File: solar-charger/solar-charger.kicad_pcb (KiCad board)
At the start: 2 copper layers, 20.8 x 10 mm, 11 parts, among them IC1 TLV809, IC2 TLV803, J1 solar, J2 battery, J3 out, Q1 AO3415, Q2 AO3416

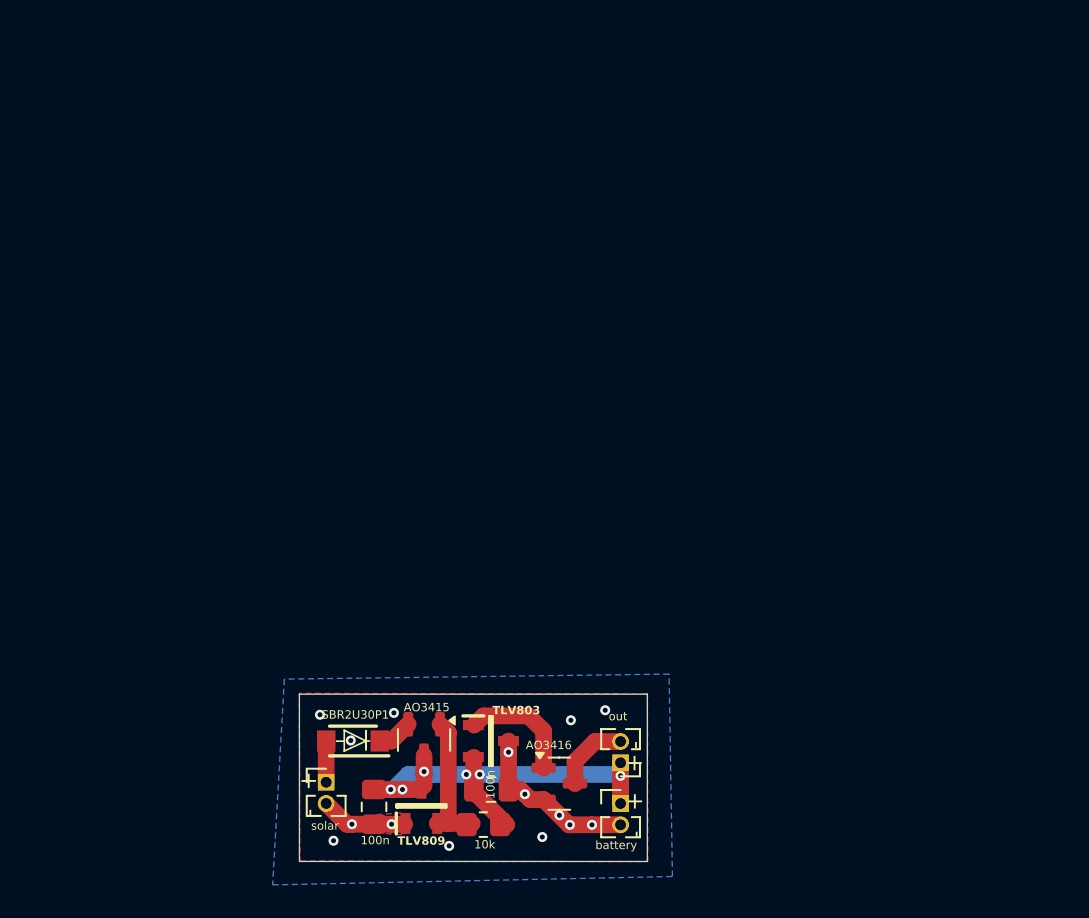
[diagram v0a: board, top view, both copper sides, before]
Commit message: finish 1. working PCB
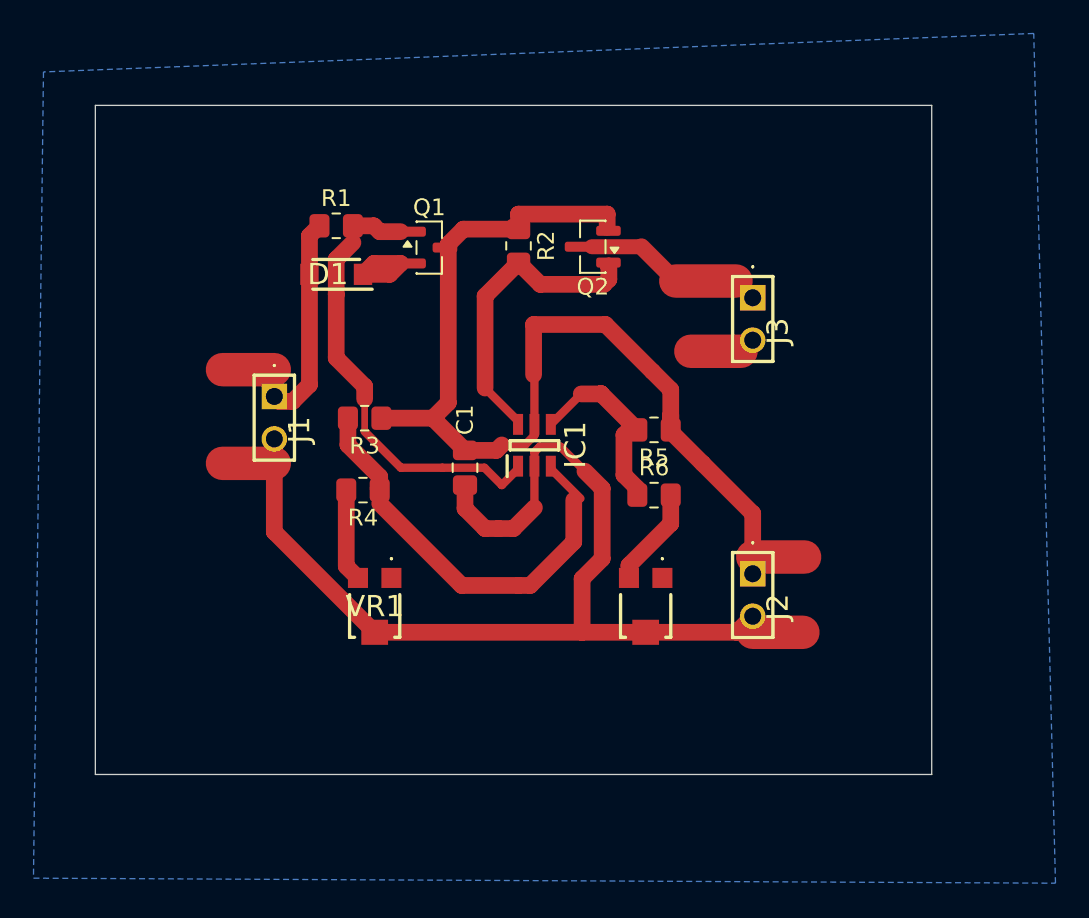
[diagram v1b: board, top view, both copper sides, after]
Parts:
- removed C2: 100n, Capacitor_SMD:C_0805_2012Metric_Pad1.18x1.45mm_HandSolder
- removed IC2: TLV803, Marcus_Library:SOT95P237X112-3N
- added R2: 51k, Resistor_SMD:R_0805_2012Metric_Pad1.20x1.40mm_HandSolder, F.Cu at (75.1, 58.7)
- added R3: 470k, Resistor_SMD:R_0805_2012Metric_Pad1.20x1.40mm_HandSolder, F.Cu at (65.9, 69.0)
- added R4: 33k, Resistor_SMD:R_0805_2012Metric_Pad1.20x1.40mm_HandSolder, F.Cu at (65.8, 73.3)
- added R5: 470k, Resistor_SMD:R_0805_2012Metric_Pad1.20x1.40mm_HandSolder, F.Cu at (83.2, 69.7)
- added R6: 33k, Resistor_SMD:R_0805_2012Metric_Pad1.20x1.40mm_HandSolder, F.Cu at (83.2, 73.6)
- added VR1: 50k, Marcus-PCB-Library:TC33X2104E, F.Cu at (66.5, 80.3)
- added VR2: 50k, Marcus-PCB-Library:TC33X2104E, F.Cu at (82.7, 80.3)
- C1: value 100n -> 100nF
- D1: value SBR2U30P1 -> SBR2U30P1-7; footprint Marcus_Library:SODFL3718X100N -> Marcus-PCB-Library:SODFL3718X100N
- IC1: value TLV809 -> TPS3700DDCR; footprint Marcus_Library:SOT95P237X95-3N -> Marcus-PCB-Library:SOT98P280X110-6N
- J1: value solar -> Solar Cell; footprint Connector_PinHeader_1.27mm:PinHeader_1x02_P1.27mm_Vertical -> Marcus-PCB-Library:10129378902001BLF
- J2: value battery -> Battery; footprint Connector_PinHeader_1.27mm:PinHeader_1x02_P1.27mm_Vertical -> Marcus-PCB-Library:10129378902001BLF
- J3: value out -> power out; footprint Connector_PinHeader_1.27mm:PinHeader_1x02_P1.27mm_Vertical -> Marcus-PCB-Library:10129378902001BLF
- Q2: value AO3416 -> AO3415
- R1: value 10k -> 51k
- moved R1 36.9 mm to (64.2, 57.5), turned to 0 degrees
- moved Q2 32.2 mm to (79.5, 58.8), turned to 180 degrees
- moved Q1 29.4 mm to (69.8, 58.8), turned to 0 degrees
- moved J3 28.9 mm to (89.1, 61.8), turned to -90 degrees
- moved D1 27.9 mm to (64.2, 60.4)
- moved J1 23.3 mm to (60.5, 67.7), turned to -90 degrees
- moved IC1 22.6 mm to (76.0, 70.6)
- moved C1 21.0 mm to (71.9, 72.0)
- moved J2 15.8 mm to (89.1, 78.3), turned to -90 degrees
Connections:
- IC1 pad 1: -BATT -> Net-(IC1-OUTA)
- IC1 pad 2: Net-(IC1-~{RESET}) -> -BATT
- IC1 pad 3: +BATT -> Net-(IC1-INA+)
- J3 pad 1: +BATT -> Net-(Q2-D)
- J3 pad 2: Net-(J3-Pin_2) -> -BATT
- Q1 pad 1: Net-(IC1-~{RESET}) -> Net-(IC1-OUTA)
- Q2 pad 1: Net-(IC2-~{RESET}) -> Net-(IC1-OUTB)
- Q2 pad 2: -BATT -> +BATT
- Q2 pad 3: Net-(J3-Pin_2) -> Net-(Q2-D)
- R1 pad 1: +BATT -> Net-(D1-A)
- R1 pad 2: Net-(IC1-~{RESET}) -> Net-(IC1-OUTA)
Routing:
- net -BATT: track 15.7 -> 73.7 mm, vias 15 -> 0
- net +BATT: track 27.7 -> 66.3 mm, vias 6 -> 0
- net Net-(IC1-OUTA): track 0.00 -> 28.2 mm
- net Net-(IC1-INA+): track 0.00 -> 25.9 mm
- net Net-(IC1-OUTB): track 0.00 -> 18.2 mm
- net Net-(D1-A): track 2.47 -> 17.1 mm
- net Net-(IC1-INB-): track 0.00 -> 11.7 mm
- net Net-(Q2-D): track 0.00 -> 10.9 mm
- net Net-(IC1-~{RESET}): track 8.96 -> 0.00 mm
- net Net-(IC2-~{RESET}): track 7.00 -> 0.00 mm
- net Net-(VR2-CW): track 0.00 -> 6.14 mm
- net Net-(VR1-CW): track 0.00 -> 5.54 mm
- net Net-(J3-Pin_2): track 4.54 -> 0.00 mm
- net Net-(D1-K): track 2.11 -> 5.04 mm
- removed copper zone on F.Cu, net -BATT
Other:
- board size 20.8 x 10 mm -> 50 x 40 mm
- board text removed: "+"
- board text removed: "-"
